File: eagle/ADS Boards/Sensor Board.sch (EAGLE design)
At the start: 19 parts, among them J1 S2B-PH-SM4-TB(LF)(SN), J2 S2B-PH-SM4-TB(LF)(SN), J3 S2B-PH-SM4-TB(LF)(SN), J4 S2B-PH-SM4-TB(LF)(SN), J5 S2B-PH-SM4-TB(LF)(SN), J6 S2B-PH-SM4-TB(LF)(SN)

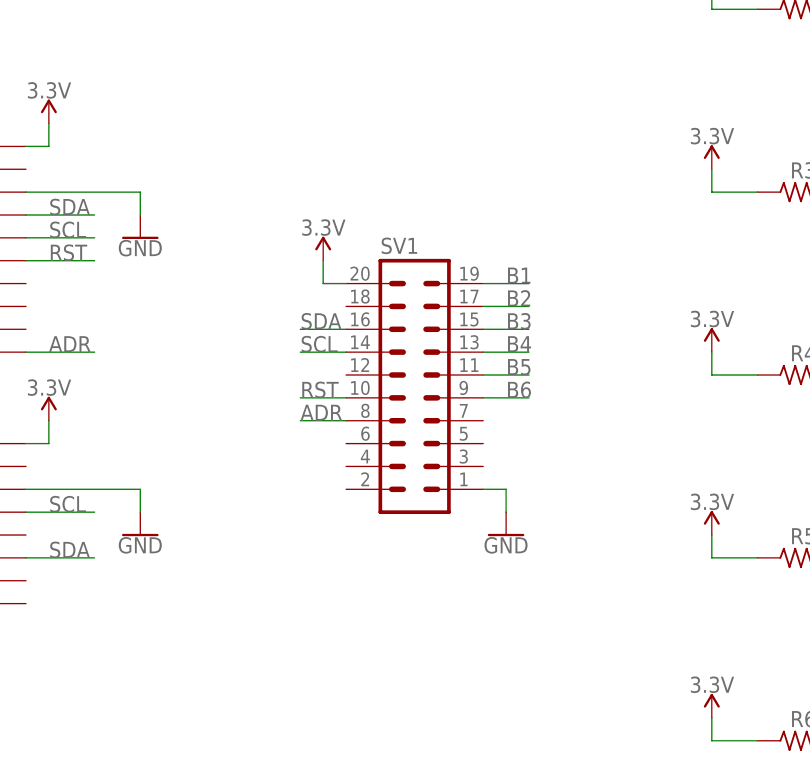
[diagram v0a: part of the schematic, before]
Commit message: Finalized Boards, Gerbers, and DXF files.
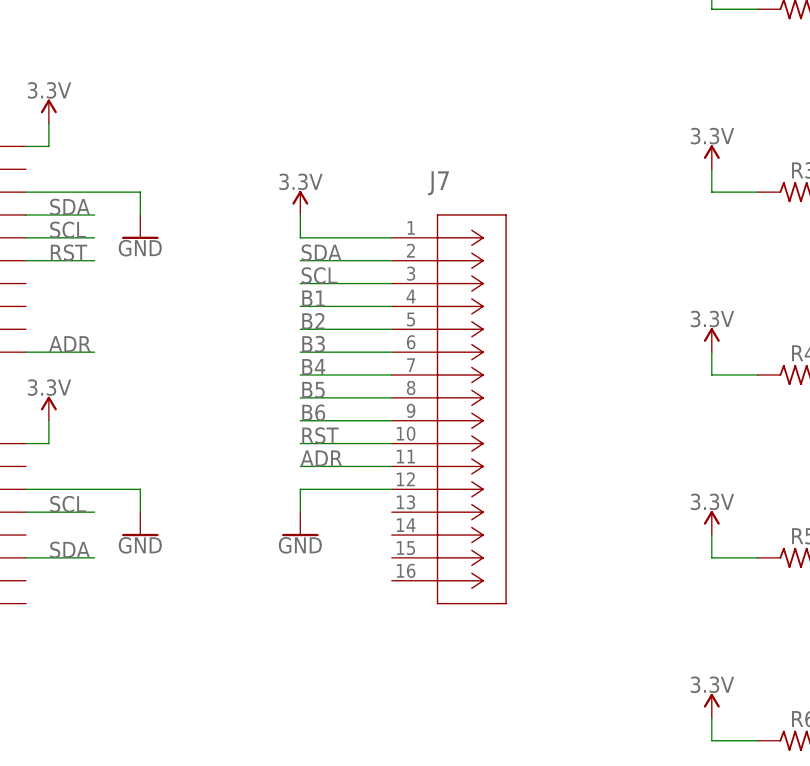
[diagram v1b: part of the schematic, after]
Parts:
- removed SV1: (no value), con-lstb:MA10-2
- added J7: 62674-121121ALF, NUSTARS ADS Library:62674-121121ALF
- R1, R2, R3, R4, R5, R6: device resistor:R-US_M1206 -> resistor:R-US_R0805
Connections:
- net 3.3V: now also J7.11; no longer SV1.20
- net ADR: now also J7.1111; no longer SV1.8
- net B1: now also J7.44; no longer SV1.19
- net B2: now also J7.55; no longer SV1.17
- net B3: now also J7.66; no longer SV1.15
- net B4: now also J7.77; no longer SV1.13
- net B5: now also J7.88; no longer SV1.11
- net B6: now also J7.99; no longer SV1.9
- net GND: now also J7.1212; no longer SV1.1
- net RST: now also J7.1010; no longer SV1.10
- net SCL: now also J7.33; no longer SV1.14
- net SDA: now also J7.22; no longer SV1.16
